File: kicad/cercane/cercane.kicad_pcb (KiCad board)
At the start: 2 copper layers, 74.9 x 33 mm, 4 parts, among them J1 Conn_02x03_Odd_Even, U1 ATtiny45-20PU, U2 NRF24L01_Breakout

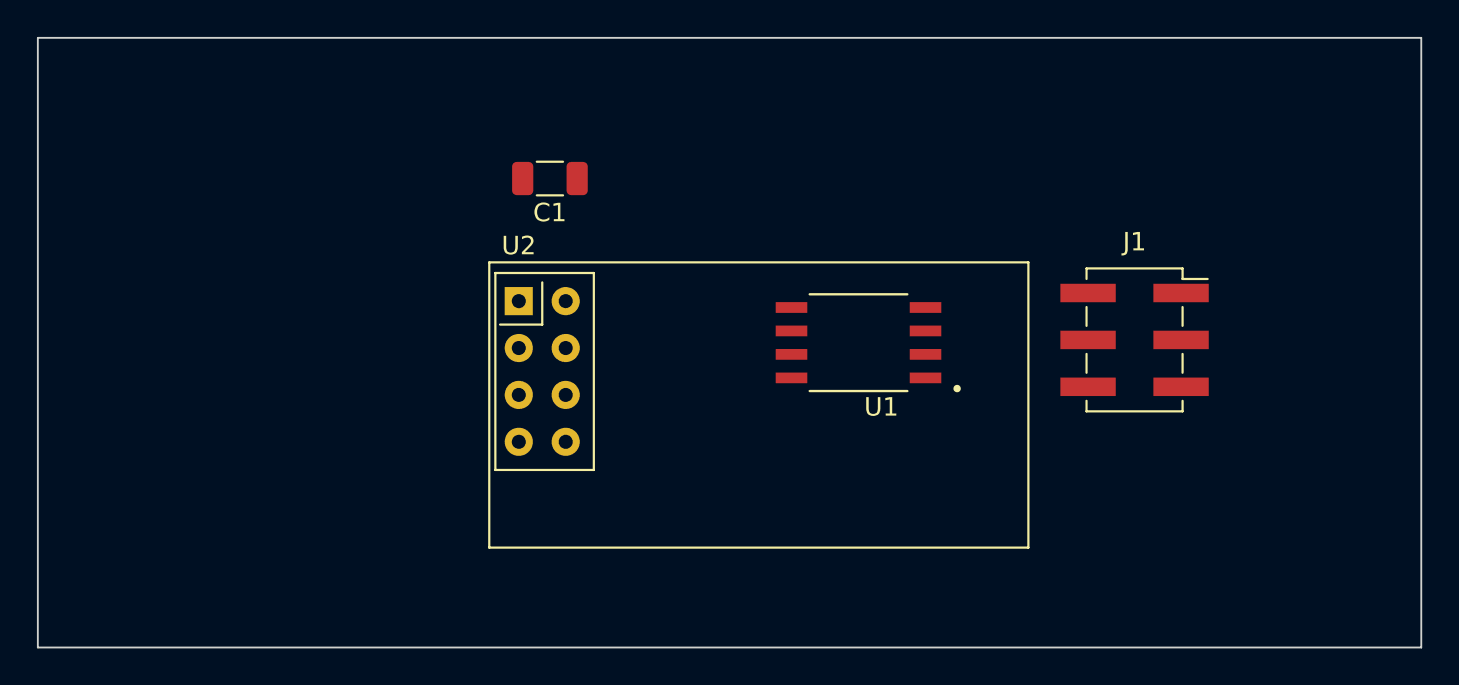
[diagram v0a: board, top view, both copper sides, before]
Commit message: Exported PCB in png and svg
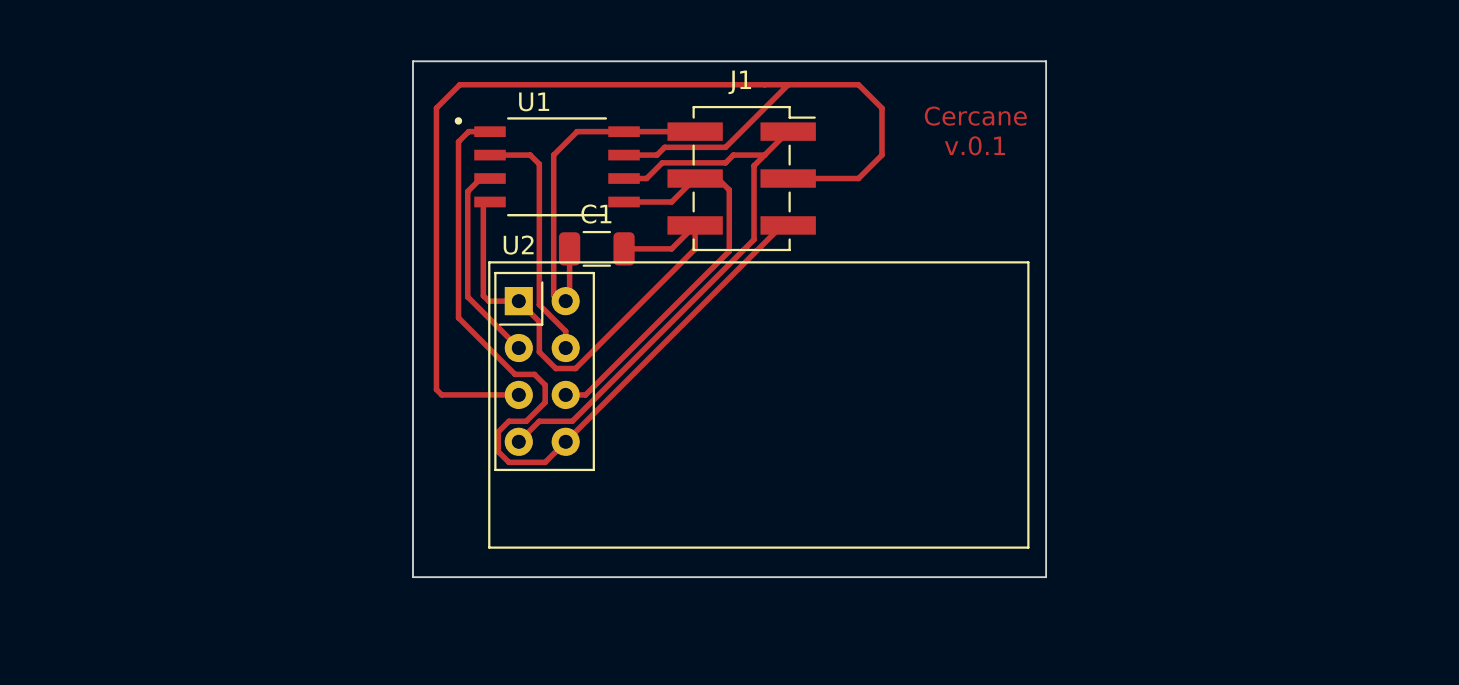
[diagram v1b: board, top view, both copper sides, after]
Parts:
- moved J1 23.0 mm to (149.9, 62.2)
- moved U1 18.9 mm to (139.9, 61.6), turned to 0 degrees
- moved C1 4.58 mm to (142.0, 66.0), turned to 0 degrees
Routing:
- net /SCK: track 0.00 -> 63.6 mm
- net /RST: track 0.00 -> 44.1 mm
- net /MISO: track 0.00 -> 32.0 mm
- net GND: track 0.00 -> 27.8 mm
- net /MOSI: track 0.00 -> 21.9 mm
- net +3V3: track 0.00 -> 19.5 mm
- net Net-(U1-Pad2): track 0.00 -> 13.4 mm
- net Net-(U1-Pad3): track 0.00 -> 11.1 mm
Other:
- board size 74.9 x 33 mm -> 34.3 x 27.9 mm
- net class Default: trace_width 0.4 -> 0.3
- board text added: "Cercane v.0.1"
